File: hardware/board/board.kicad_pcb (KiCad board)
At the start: 4 copper layers, 45 x 80 mm, 177 parts, among them J2 Conn_01x26_MountingPin, J3 Conn_01x26_MountingPin, J4 Conn_01x26_MountingPin, J5 Conn_01x03, Q1 AO3400A, Q2 AO3400A, Q3 AO3400A, SW1 SW_Push, SW2 SW_Push, SW3 SKRTLAE010, U1 STM32WB55RGV6, U10 74HC4051, U11 74HC4051, U12 74HC4051, U13 SN74LV1T125DCKR, U14 USBLC6-2P6, U15 FAN48610BUC50X, U16 RS3221-3.3YUTDN4, U6 COS8054TR, U7 74HC4051, U8 74HC4051, U9 74HC4051, X1 XL7EL89CKI-111YLC-32M, X2 FC-12M32.768KHZ7PF20PPM

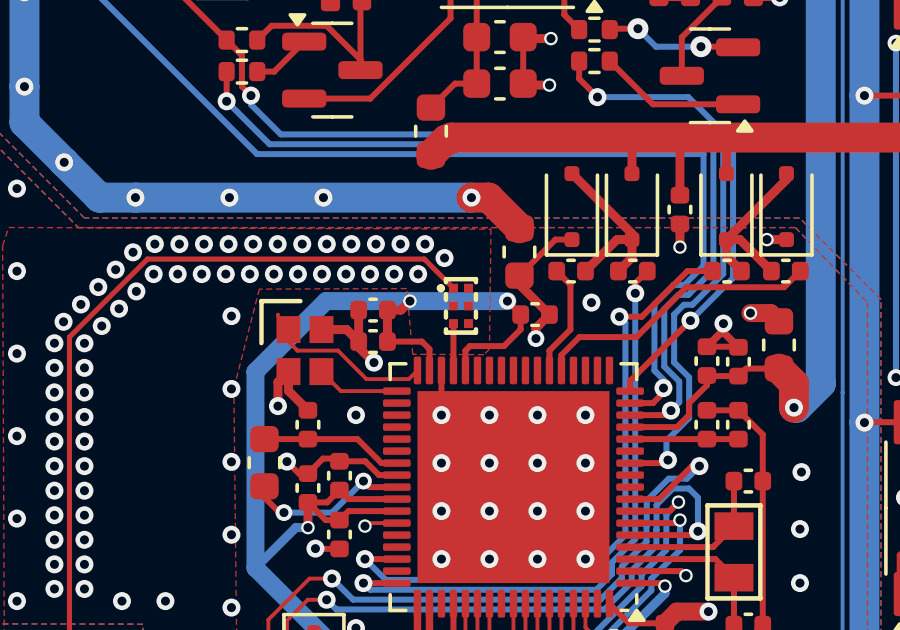
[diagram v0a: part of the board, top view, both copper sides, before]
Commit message: impdance matching
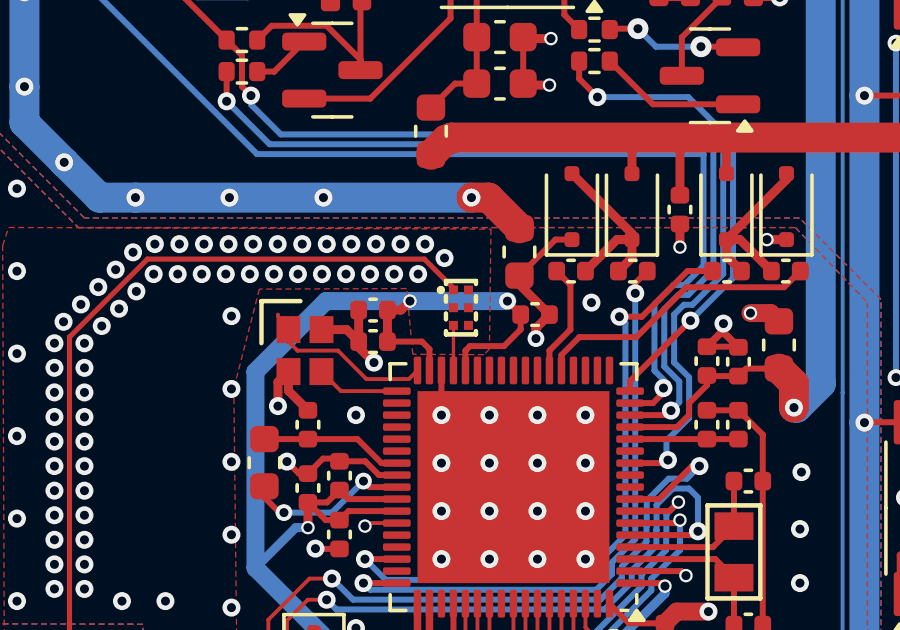
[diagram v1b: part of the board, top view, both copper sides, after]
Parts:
- moved FL2 0.06 mm to (73.2, 133.1)
